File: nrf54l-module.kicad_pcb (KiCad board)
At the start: 6 copper layers, 16 x 25 mm, 138 parts, among them SW1 TS24CA, SW2 TD-1183SN-1.7H-250, U1 NRF54L15-QFAA-R, U2 XL-0201SURC, U4 XL-0201SURC, U5 XL-0201SURC, U6 TLV62569DRLR, X1 XL7EL89CKI-111YLC-32M

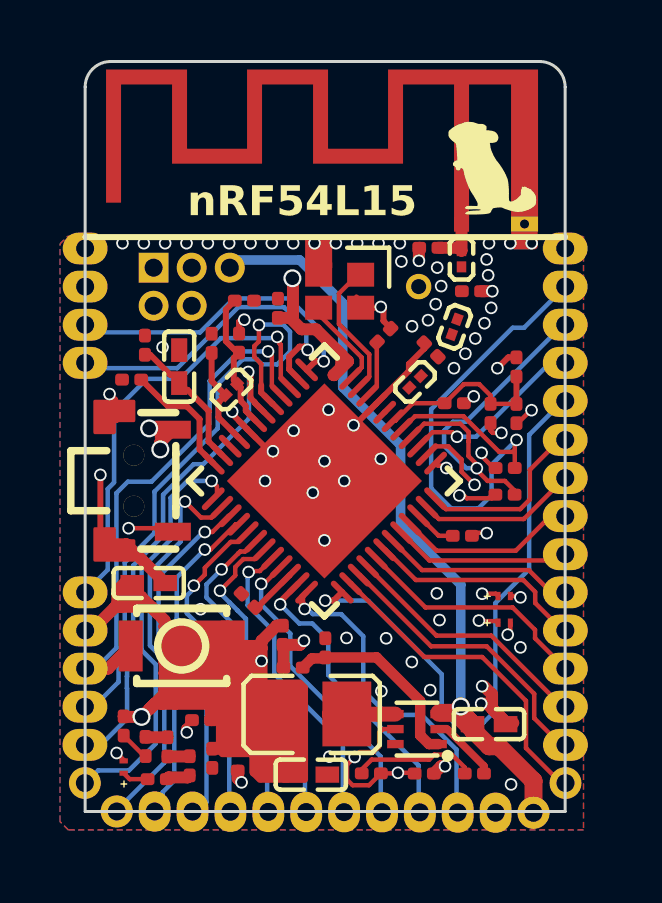
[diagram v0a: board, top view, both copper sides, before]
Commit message: chore: refactoring
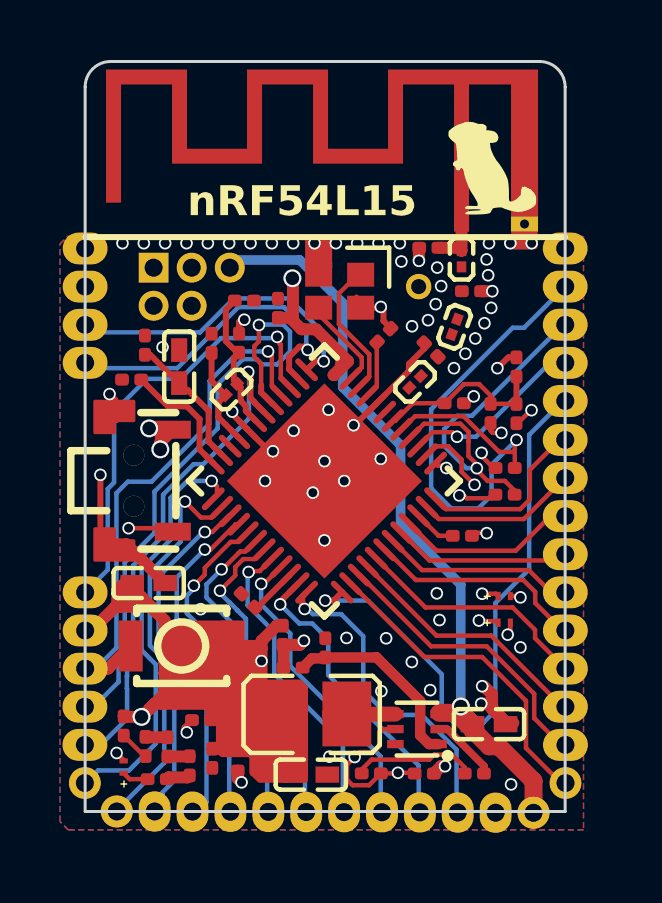
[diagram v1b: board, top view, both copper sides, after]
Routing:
- net GND: track 35.3 -> 39.9 mm

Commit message: chore: checkpoint
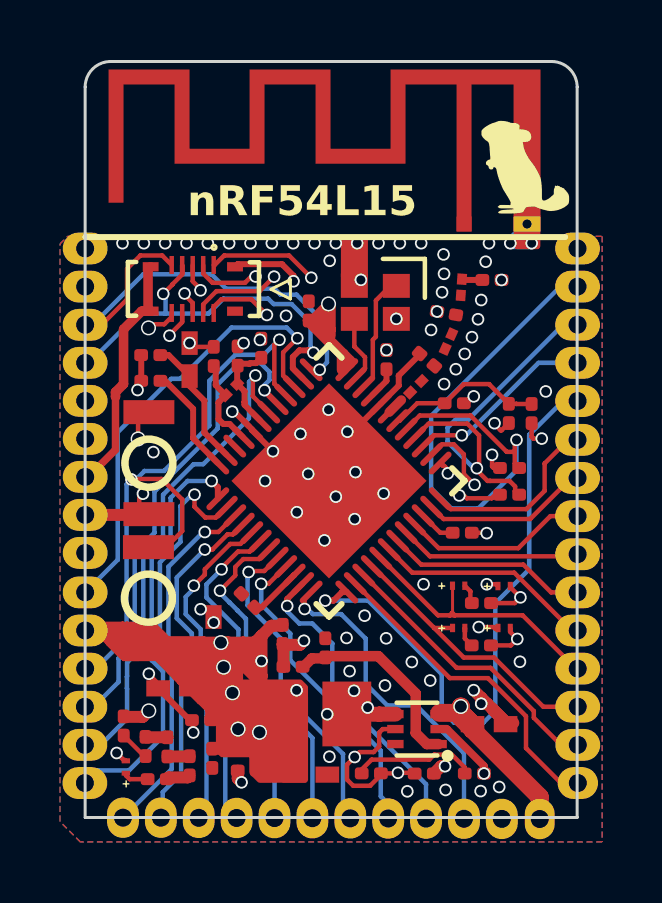
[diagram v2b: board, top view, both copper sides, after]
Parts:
- removed the ? at (28.1, 28.4)
- removed the ? at (36.9, 27.8)
- removed the ? at (29.4, 28.4)
- removed the ? at (29.4, 27.1)
- removed the ? at (28.1, 27.1)
- removed the ? at (30.6, 27.1)
- removed C13: 1.5pF, Capacitor_SMD:C_0201_0603Metric
- removed kibuzzard-68448B88: G***, kibuzzard-68448B88
- removed kibuzzard-68449000: G***, kibuzzard-68449000
- removed kibuzzard-6846144B: G***, kibuzzard-6846144B
- removed kibuzzard-68461451: G***, kibuzzard-68461451
- removed kibuzzard-68461457: G***, kibuzzard-68461457
- removed kibuzzard-684616DE: G***, kibuzzard-684616DE
- removed kibuzzard-6846173A: G***, kibuzzard-6846173A
- removed kibuzzard-68461772: G***, kibuzzard-68461772
- removed kibuzzard-68461788: G***, kibuzzard-68461788
- removed kibuzzard-68463A73: G***, kibuzzard-68463A73
- removed kibuzzard-68463A78: G***, kibuzzard-68463A78
- removed kibuzzard-68463A7B: G***, kibuzzard-68463A7B
- removed kibuzzard-68463A81: G***, kibuzzard-68463A81
- removed kibuzzard-68463A85: G***, kibuzzard-68463A85
- added ?: , , F.Cu at (25.8, 36.6)
- added ?: , , F.Cu at (25.8, 32.8)
- added ?: , , F.Cu at (25.8, 35.4)
- added ?: , , F.Cu at (25.8, 31.6)
- added ?: , , F.Cu at (25.8, 34.1)
- added C23: 10uF, easyeda2kicad:C0402, F.Cu at (30.1, 39.3)
- added J1: BM28B0.6-10DS/2-0.35V(51), easyeda2kicad:CONN-SMD_BM28B0.6-10DS-2-0.35V-51, F.Cu at (29.4, 27.8)
- added R15: 1kΩ, Resistor_SMD:R_0201_0603Metric, F.Cu at (39.0, 38.3)
- added R16: 1kΩ, Resistor_SMD:R_0201_0603Metric, F.Cu at (39.0, 39.7)
- added U3: XL-0201SURC, easyeda2kicad:LED-SMD_L0.65-W0.35-P0.41_XL-0201SURC, F.Cu at (38.3, 37.7)
- added U7: XL-0201SURC, easyeda2kicad:LED-SMD_L0.65-W0.35-P0.41_XL-0201SURC, F.Cu at (38.3, 39.1)
- added kibuzzard-68478C96: G***, kibuzzard-68478C96, B.Cu at (27.8, 29.1)
- added kibuzzard-68478D5A: G***, kibuzzard-68478D5A, B.Cu at (27.3, 26.5)
- added kibuzzard-68478D5E: G***, kibuzzard-68478D5E, B.Cu at (28.4, 27.8)
- added kibuzzard-68478D64: G***, kibuzzard-68478D64, B.Cu at (27.8, 31.6)
- added kibuzzard-68478D6B: G***, kibuzzard-68478D6B, B.Cu at (27.8, 32.8)
- added kibuzzard-68478D71: G***, kibuzzard-68478D71, B.Cu at (27.2, 34.1)
- added kibuzzard-68478D74: G***, kibuzzard-68478D74, B.Cu at (27.2, 35.4)
- added kibuzzard-68478D78: G***, kibuzzard-68478D78, B.Cu at (27.8, 36.6)
- added kibuzzard-68478D82: G***, kibuzzard-68478D82, B.Cu at (27.8, 38.0)
- added kibuzzard-68478D86: G***, kibuzzard-68478D86, B.Cu at (27.3, 39.2)
- added kibuzzard-68478D8D: G***, kibuzzard-68478D8D, B.Cu at (27.8, 40.5)
- added kibuzzard-68478D98: G***, kibuzzard-68478D98, B.Cu at (27.8, 41.8)
- added kibuzzard-68478D9B: G***, kibuzzard-68478D9B, B.Cu at (27.8, 43.1)
- L2, L3: value LQP03TN3N5B02D -> MLG0603P2N7CT000
- SW1: value TS24CA -> ~; footprint easyeda2kicad:SW-SMD_TS24CA -> easyeda2kicad:KEY-SMD_B3U-1000PM
- SW2: value TD-1183SN-1.7H-250 -> ~
- moved G*** 11.2 mm to (28.8, 23.1)
- moved kibuzzard-6844924F 4.73 mm to (33.9, 33.9)
- moved kibuzzard-68449253 4.73 mm to (36.3, 34.5)
- moved kibuzzard-684623CD 4.73 mm to (35.1, 34.5)
- moved kibuzzard-68449359 4.32 mm to (32.1, 38.5)
- moved kibuzzard-68449351 4.32 mm to (34.5, 38.5)
- moved kibuzzard-68449360 4.32 mm to (33.3, 38.5)
- moved C18 3.61 mm to (28.8, 41.2), turned to 180 degrees
- moved C7 2.36 mm to (39.4, 27.5), turned to 0 degrees
- moved SW2 1.94 mm to (27.9, 38.1), turned to 90 degrees
- moved C5 1.86 mm to (30.9, 30.1), turned to -90 degrees
- moved X1 1.25 mm to (35.5, 28.3)
- moved C8 1.11 mm to (37.9, 28.6), turned to 170 degrees
- moved G*** 1.10 mm to (40.4, 23.8)
- moved C11 1.03 mm to (33.3, 28.6)
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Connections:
- AE1 pad 2: (no net) -> GND
- SW1 pad 1: GND -> +1V8
- SW1 pad 2: GND -> nRESET
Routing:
- net P0.04: track 18.9 -> 38.3 mm, vias 1 -> 2
- net P0.02: track 6.39 -> 25.1 mm, vias 1 -> 2
- net P0.03: track 12.8 -> 31.3 mm, vias 1 -> 2
- net +1V8: track 90.6 -> 109.1 mm, vias 5 -> 11
- net SWDCLK: track 15.0 -> 32.8 mm, vias 1 -> 3
- net SWDIO: track 12.5 -> 26.5 mm, vias 1 -> 2
- net VIN: track 29.7 -> 39.6 mm
- net GND: track 39.9 -> 32.0 mm, vias 67 -> 80
- net P1.11: track 14.7 -> 21.3 mm, vias 1 -> 2
- net P1.09: track 10.5 -> 16.0 mm
- net P1.13: track 20.8 -> 16.5 mm
- net nRESET: track 41.1 -> 44.8 mm, vias 2 -> 3
- net SW_EN: track 26.8 -> 23.7 mm
- net P1.12: track 18.2 -> 21.2 mm, vias 1 -> 2
- net P1.10: track 10.9 -> 13.6 mm, vias 1 -> 2
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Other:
- board size 16 x 25 mm -> 16.4 x 25.2 mm
- board text added: "16"
- board text added: "2.5V ≤ VIN ≤ 5.5V"
- board text removed: "01"
- board text removed: "1.8V ≤ VIN ≤ 5.5V"

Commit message: chore: checkpoint
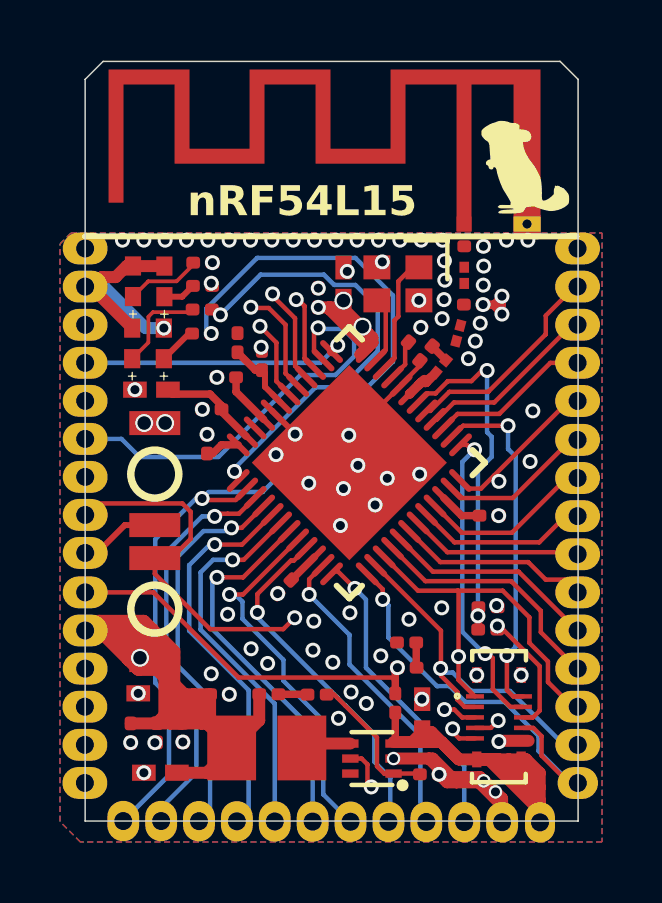
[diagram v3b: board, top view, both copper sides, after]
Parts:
- removed the C14 at (38.1, 31.6)
- removed FB1: BLM03PX121SN1D, easyeda2kicad:L0201
- removed R12, R13, R14, R15, R16: 1kΩ, Resistor_SMD:R_0201_0603Metric
- removed the R2 at (28.2, 44.2)
- removed the U2 at (27.2, 43.8)
- removed U3, U4, U5, U7: XL-0201SURC, easyeda2kicad:LED-SMD_L0.65-W0.35-P0.41_XL-0201SURC
- removed kibuzzard-68448BA2: G***, kibuzzard-68448BA2
- removed kibuzzard-68448DE0: G***, kibuzzard-68448DE0
- removed kibuzzard-68448DE9: G***, kibuzzard-68448DE9
- removed kibuzzard-68448E11: G***, kibuzzard-68448E11
- removed kibuzzard-68448E3B: G***, kibuzzard-68448E3B
- removed kibuzzard-68448E4C: G***, kibuzzard-68448E4C
- removed kibuzzard-68448E55: G***, kibuzzard-68448E55
- removed kibuzzard-684495B0: G***, kibuzzard-684495B0
- removed kibuzzard-684495B4: G***, kibuzzard-684495B4
- removed kibuzzard-684495B8: G***, kibuzzard-684495B8
- removed kibuzzard-684617E6: G***, kibuzzard-684617E6
- removed kibuzzard-684623E2: G***, kibuzzard-684623E2
- removed kibuzzard-68478C96: G***, kibuzzard-68478C96
- removed kibuzzard-68478D64: G***, kibuzzard-68478D64
- removed kibuzzard-68478D6B: G***, kibuzzard-68478D6B
- removed kibuzzard-68478D74: G***, kibuzzard-68478D74
- removed kibuzzard-68478D78: G***, kibuzzard-68478D78
- removed kibuzzard-68478D82: G***, kibuzzard-68478D82
- added C11: 2.2uF, Capacitor_SMD:C_0201_0603Metric, F.Cu at (30.3, 41.4)
- added LED1: TZ-P2-0402RTIA1-0.45T, easyeda2kicad:LED0402-RD_RED, F.Cu at (27.4, 27.6)
- added LED2: TZ-P2-0402RTIA1-0.45T, easyeda2kicad:LED0402-RD_RED, F.Cu at (28.4, 27.6)
- added LED3: TZ-P2-0402RTIA1-0.45T, easyeda2kicad:LED0402-RD_RED, F.Cu at (27.4, 29.7)
- added LED4: TZ-P2-0402RTIA1-0.45T, easyeda2kicad:LED0402-RD_RED, F.Cu at (28.4, 29.7)
- added R10: 1kΩ, Resistor_SMD:R_0201_0603Metric, F.Cu at (29.7, 28.5)
- added kibuzzard-684F74F9: G***, kibuzzard-684F74F9, B.Cu at (27.8, 29.1)
- added kibuzzard-684F750C: G***, kibuzzard-684F750C, B.Cu at (27.8, 30.3)
- added kibuzzard-684F751D: G***, kibuzzard-684F751D, B.Cu at (27.8, 31.6)
- added kibuzzard-684F753F: G***, kibuzzard-684F753F, B.Cu at (27.8, 32.8)
- added kibuzzard-684F7560: G***, kibuzzard-684F7560, B.Cu at (27.8, 35.4)
- added kibuzzard-684F7579: G***, kibuzzard-684F7579, B.Cu at (27.8, 36.6)
- added kibuzzard-684F7581: G***, kibuzzard-684F7581, B.Cu at (27.8, 38.0)
- added kibuzzard-684F75DA: G***, kibuzzard-684F75DA, B.Cu at (40.3, 44.3)
- added kibuzzard-684F75DE: G***, kibuzzard-684F75DE, B.Cu at (40.2, 43.0)
- added kibuzzard-684F75E1: G***, kibuzzard-684F75E1, B.Cu at (40.2, 41.8)
- added kibuzzard-684F75E4: G***, kibuzzard-684F75E4, B.Cu at (40.2, 40.5)
- added kibuzzard-684F75E9: G***, kibuzzard-684F75E9, B.Cu at (40.2, 39.2)
- added kibuzzard-684F75ED: G***, kibuzzard-684F75ED, B.Cu at (40.2, 38.0)
- added kibuzzard-684F75F1: G***, kibuzzard-684F75F1, B.Cu at (40.2, 36.7)
- added kibuzzard-684F75F7: G***, kibuzzard-684F75F7, B.Cu at (40.2, 35.4)
- added kibuzzard-684F75FF: G***, kibuzzard-684F75FF, B.Cu at (40.2, 34.1)
- added kibuzzard-684F7617: G***, kibuzzard-684F7617, B.Cu at (40.2, 32.9)
- added kibuzzard-684F761F: G***, kibuzzard-684F761F, B.Cu at (40.3, 31.6)
- moved J1 17.6 mm to (39.6, 42.1), turned to -90 degrees
- moved C14 16.4 mm to (34.4, 27.7), turned to 90 degrees
- moved R11 14.4 mm to (29.7, 29.3), turned to 0 degrees
- moved R7 12.8 mm to (29.7, 27.0)
- moved R9 11.9 mm to (29.7, 27.7)
- moved R8 7.24 mm to (39.2, 39.2), turned to 0 degrees
- moved C20 6.62 mm to (39.2, 38.4), turned to 0 degrees
- moved R5 5.46 mm to (37.3, 44.0), turned to 0 degrees
- moved R6 4.92 mm to (36.5, 39.6), turned to 180 degrees
- moved R4 3.72 mm to (36.5, 40.5), turned to 0 degrees
- moved C7 2.85 mm to (28.3, 44.0)
- moved C13 2.82 mm to (29.9, 33.0), turned to 90 degrees
- moved C5 2.80 mm to (28.1, 41.3), turned to 180 degrees
- moved C9 2.73 mm to (30.0, 31.9)
- moved R2 2.54 mm to (36.1, 41.6), turned to -90 degrees
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- renumbered C12 to C1, C19 to C10, C20 to C12, C10 to C13, C22 to C14, C11 to C15, C2 to C16, C6 to C17, C8 to C18, C7 to C19, C1 to C2, C15 to C20, C16 to C21, C9 to C22, C5 to C3, C17 to C4, C23 to C5, C4 to C6, C18 to C7, C21 to C8, C3 to C9, L4 to L1, L1 to L2, L2 to L3, L3 to L4, R3 to R1, R6 to R2, R4 to R3, R9 to R4, R10 to R6, R8 to R7, R1 to R8, R7 to R9, U6 to U1, U1 to U2
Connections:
- ? pad 1: P0.00 -> P2.10
- ? pad 1: P0.01 -> P0.00
- ? pad 1: P2.10 -> P2.09
- ? pad 1: P2.05 -> P2.04
- ? pad 1: SW_EN -> nRESET
- ? pad 1: SWDIO -> P1.10
- ? pad 1: P2.09 -> P2.08
- ? pad 1: P2.02 -> P0.01
- ? pad 1: P2.03 -> P2.02
- ? pad 1: P2.07 -> P2.06
- ? pad 1: P1.09 -> SWDCLK
- ? pad 1: nRESET -> P1.11
- ? pad 1: P2.06 -> P2.05
- ? pad 1: P2.04 -> P2.03
- ? pad 1: SWDCLK -> SWDIO
- ? pad 1: P1.10 -> P1.09
- ? pad 1: P1.11 -> SW_EN
- ? pad 1: P2.08 -> P2.07
- J1 pad 1: P0.04 -> P2.04
- J1 pad 2: P0.03 -> P2.03
- J1 pad 3: P0.02 -> P1.05
- J1 pad 4: P1.10 -> P1.06
- J1 pad 5: P1.09 -> P1.07
- J1 pad 7: P1.11 -> P2.02
- R11 pad 2: Net-(R11-Pad2) -> P1.01
- R7 pad 2: P0.03 -> P0.00
- R9 pad 2: P0.04 -> P0.01
- SW2 pad 2: P1.12 -> P1.11
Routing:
- net P0.04: track 38.3 -> 7.11 mm, vias 2 -> 0
- net GND_LED: track 34.1 -> 8.27 mm, vias 2 -> 1
- net P0.03: track 31.3 -> 6.06 mm, vias 2 -> 0
- net +1V8: track 109.1 -> 86.3 mm, vias 11 -> 7
- net nRESET: track 44.8 -> 22.1 mm, vias 3 -> 1
- net P0.02: track 25.1 -> 5.37 mm, vias 2 -> 0
- net P1.01: track 14.1 -> 32.8 mm, vias 1 -> 2
- net P0.00: track 5.32 -> 22.9 mm, vias 0 -> 1
- net GND: track 32.0 -> 15.1 mm, vias 80 -> 83
- net P1.00: track 13.9 -> 29.1 mm, vias 1 -> 2
- net P0.01: track 6.50 -> 20.3 mm, vias 0 -> 2
- net P1.06: track 11.2 -> 22.9 mm, vias 1 -> 2
- net P1.05: track 10.9 -> 21.5 mm, vias 1 -> 2
- net P1.07: track 10.9 -> 19.1 mm, vias 1 -> 2
- net P2.02: track 21.4 -> 14.0 mm
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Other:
- board size 16.4 x 25.2 mm -> 16.4 x 25.3 mm
- board text added: "1665"
- board text removed: "16"
- board text removed: "65"
